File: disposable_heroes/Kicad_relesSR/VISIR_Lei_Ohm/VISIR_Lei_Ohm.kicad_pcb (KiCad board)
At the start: 2 copper layers, 95.3 x 90.1 mm, 32 parts, among them J1 Raspberry PI5, J10 Amperimetro+, J11 Amperimetro-, J2 Fonte dc_VB, J3 12V, J4 Voltimetro+, J5 Ext_OUT_PI, J6 Ext_OUT_PI, J7 Ext_OUT_PI, J8 Ext_OUT_PI, J9 Voltimetro-, K1 3572-1220-123, K2 3572-1220-123, K3 3572-1220-123, K4 3570-1331-123, K5 3570-1331-123, K6 3570-1331-123, K7 3570-1331-123, K8 3570-1331-123, U1 74HC595N_112, U2 ULN2003, U3 ULN2003

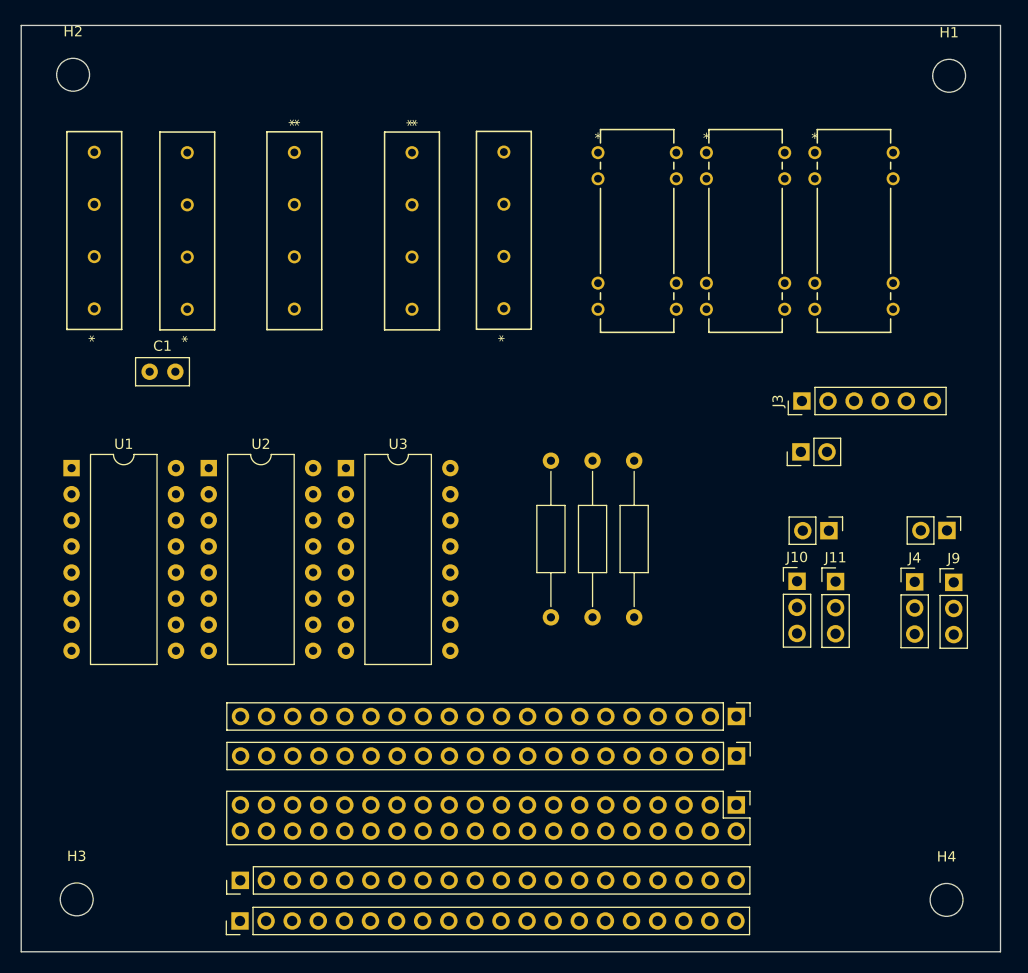
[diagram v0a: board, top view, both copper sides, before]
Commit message: update - boards done
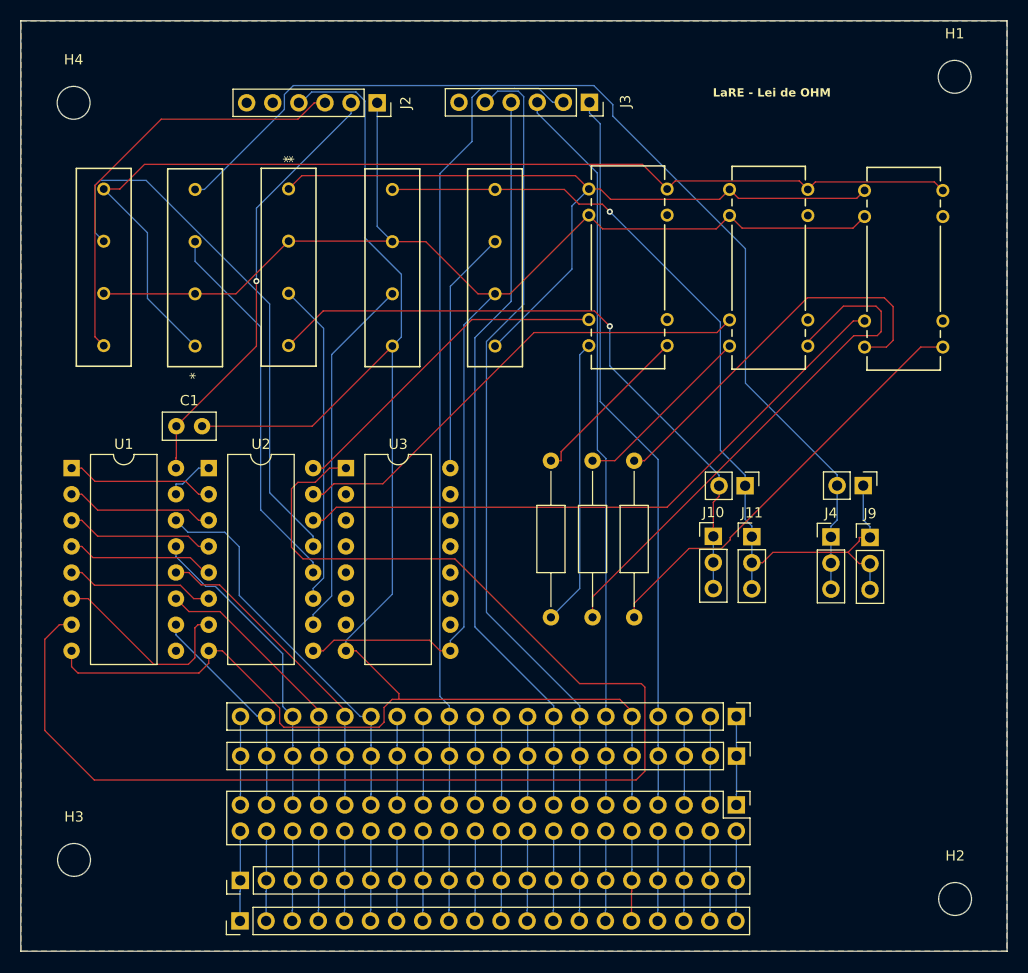
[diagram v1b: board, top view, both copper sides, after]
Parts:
- J2: value Fonte dc_VB -> Power Sources; footprint Connector_PinHeader_2.54mm:PinHeader_1x02_P2.54mm_Vertical -> Connector_PinSocket_2.54mm:PinSocket_1x06_P2.54mm_Vertical
- J3: value 12V -> PI_config; footprint Connector_PinHeader_2.54mm:PinHeader_1x06_P2.54mm_Vertical -> Connector_PinSocket_2.54mm:PinSocket_1x06_P2.54mm_Vertical
- moved H2 117.5 mm to (211.5, 115.7)
- moved H4 115.0 mm to (125.8, 38.2)
- moved J2 53.4 mm to (155.3, 38.2), turned to -90 degrees
- moved J3 35.7 mm to (175.9, 38.2), turned to -90 degrees
- moved J10 9.25 mm to (188.0, 80.4)
- moved J9 9.25 mm to (203.2, 80.5)
- moved MES3 9.25 mm to (191.1, 75.5)
- moved J11 9.25 mm to (191.8, 80.5)
- moved J4 9.25 mm to (199.4, 80.5)
- moved MES1 9.25 mm to (202.6, 75.5)
- moved K3 6.08 mm to (202.7, 46.8)
- moved C1 5.90 mm to (135.8, 69.7)
- moved K2 4.23 mm to (189.6, 46.7)
- moved K7 4.06 mm to (156.8, 46.7)
- moved H3 3.85 mm to (125.8, 111.9)
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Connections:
- C1 pad 1: /5VPower1 -> /5V
- J1 pad 11: Net-(J1-GPIO17) -> /RCLK_{filters}
- J1 pad 13: Net-(J1-GPIO27) -> /SER_{filters}
- J1 pad 15: Net-(J1-GPIO22) -> /~{OE}_{filters}
- J1 pad 23: Net-(J1-GPIO11/SCLK) -> /~{SRCLR}_{filters}
- J1 pad 7: Net-(J1-GPIO4/GPCLK0) -> /SRCLK_{filters}
- J2 pad 1: VCC -> /12V
- J2 pad 2: D -> /5V
- J3 pad 1: /12V -> /SRCLK_{filters}
- J3 pad 2: /12V -> /~{SRCLR}_{filters}
- J3 pad 3: /12V -> /RCLK_{filters}
- J3 pad 4: /12V -> /~{OE}_{filters}
- J3 pad 5: /12V -> /SER_{filters}
- J3 pad 6: /12V -> unconnected-(J3-Pin_6-Pad6)
- J7 pad 12: Net-(J1-GPIO11/SCLK) -> /~{SRCLR}_{filters}
- J7 pad 4: Net-(J1-GPIO4/GPCLK0) -> /SRCLK_{filters}
- J7 pad 6: Net-(J1-GPIO17) -> /RCLK_{filters}
- J7 pad 7: Net-(J1-GPIO27) -> /SER_{filters}
- J7 pad 8: Net-(J1-GPIO22) -> /~{OE}_{filters}
- J8 pad 12: Net-(J1-GPIO11/SCLK) -> /~{SRCLR}_{filters}
- J8 pad 4: Net-(J1-GPIO4/GPCLK0) -> /SRCLK_{filters}
- J8 pad 6: Net-(J1-GPIO17) -> /RCLK_{filters}
- J8 pad 7: Net-(J1-GPIO27) -> /SER_{filters}
- J8 pad 8: Net-(J1-GPIO22) -> /~{OE}_{filters}
- K4 pad 1: VCC -> /5V_{VB}
- K4 pad 2: unconnected-(K4-Pad2) -> /12V
- U1 pad 16: /5VPower1 -> /5V
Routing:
- net GND: track 0.00 -> 167.1 mm
- net /12V: track 0.00 -> 148.4 mm
- net /I_{21}: track 0.00 -> 132.9 mm
- net A: track 0.00 -> 103.9 mm
- net Net-(J4-Pin_1): track 0.00 -> 102.9 mm
- net C: track 0.00 -> 87.7 mm, vias 0 -> 1
- net /~{SRCLR}_{filters}: track 0.00 -> 80.4 mm
- net /SER_{filters}: track 0.00 -> 78.6 mm
- net B: track 0.00 -> 77.7 mm
- net /~{OE}_{filters}: track 0.00 -> 73.0 mm
- net /RCLK_{filters}: track 0.00 -> 71.2 mm
- net /SRCLK_{filters}: track 0.00 -> 71.2 mm
- net Net-(J10-Pin_1): track 0.00 -> 63.4 mm, vias 0 -> 1
- net /O_{13}: track 0.00 -> 61.7 mm
- net /O_{14}: track 0.00 -> 53.3 mm
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- added copper zone on B.Cu, net GND
- added copper zone on F.Cu, net GND
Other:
- board size 95.3 x 90.1 mm -> 96 x 90.5 mm
- board text added: "LaRE - Lei de OHM"
